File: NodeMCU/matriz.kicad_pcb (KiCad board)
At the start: 2 copper layers, 70 x 70 mm, 25 parts, among them J1 Conn_01x05, Q1 Q_NPN_CBE, Q2 Q_NPN_CBE, Q3 Q_NPN_CBE, SW1 SW_Push_Open, SW2 SW_Push, U3 NodeMCU1.0(ESP-12E)

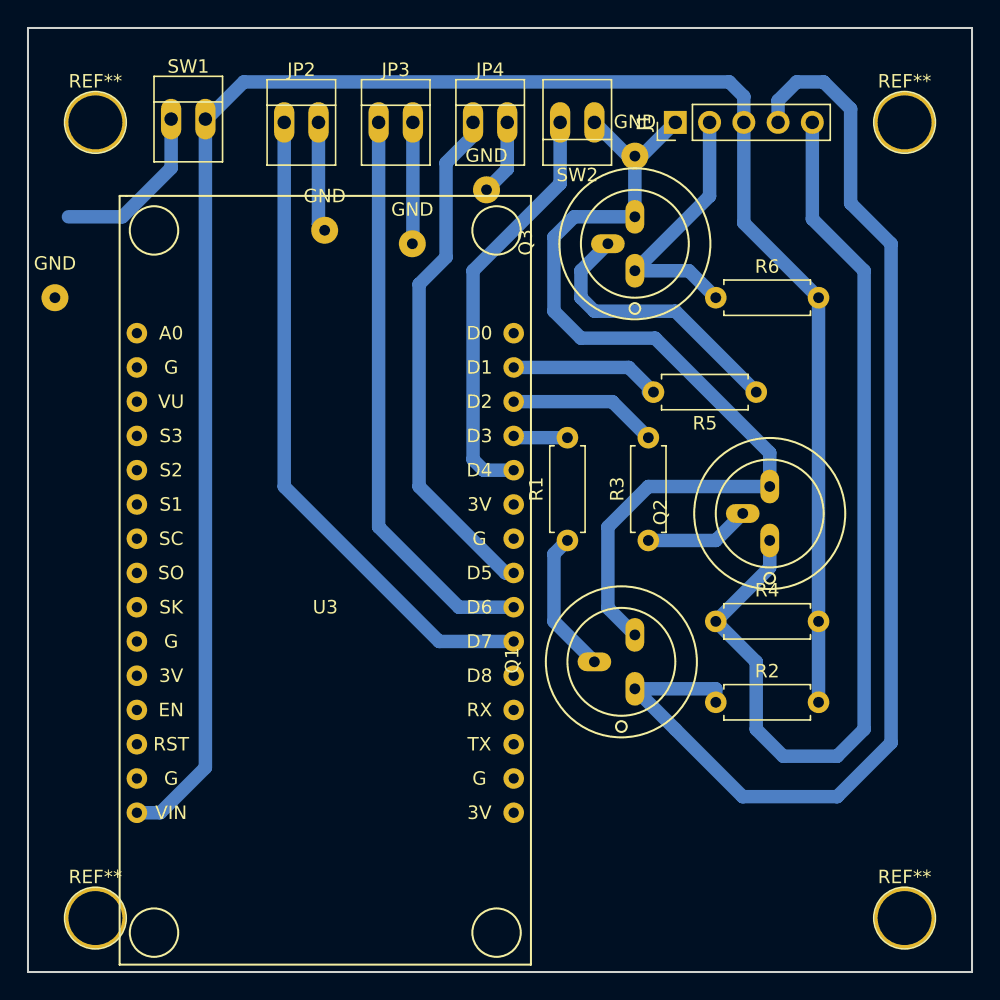
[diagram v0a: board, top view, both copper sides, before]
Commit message: Ultimos cambios
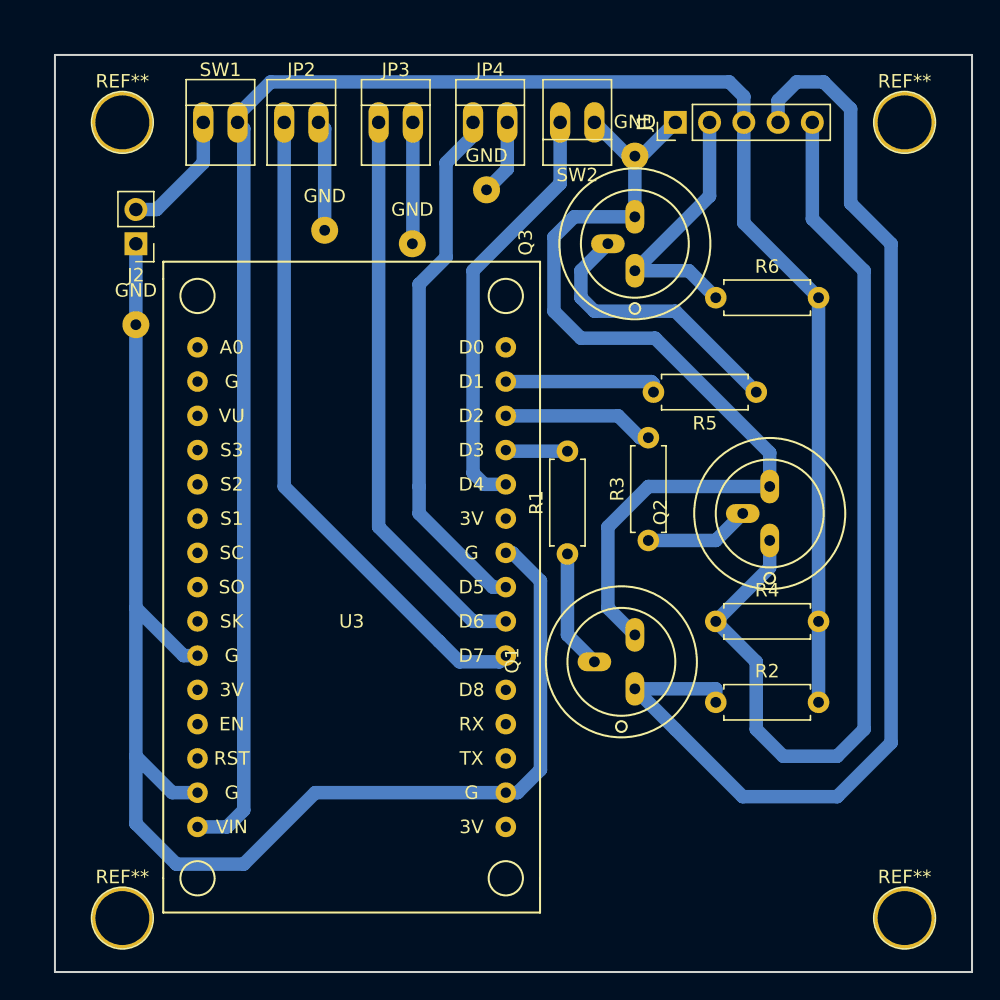
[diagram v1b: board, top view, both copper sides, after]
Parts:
- added J2: Conn_01x02, Pin_Headers:Pin_Header_Straight_1x02_Pitch2.54mm, F.Cu at (92.0, 81.0)
- U3: footprint ESP8266:NodeMCU1.0(12-E) -> lib:NodeMCU1.0(12-E)
- moved GND 6.32 mm to (92.0, 87.0)
- moved SW1 2.40 mm to (97.0, 72.0)
- moved U3 2.22 mm to (108.0, 109.0)
- moved REF** 2.00 mm to (91.0, 131.0)
- moved REF** 2.00 mm to (91.0, 72.0)
- moved R1 1.00 mm to (124.0, 104.0)
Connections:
- GND pad 1: (no net) -> /GND
- GND pad 1: GNDPWR -> /GND (x4)
- J1 pad 1: GNDPWR -> /GND
- JP2 pad 2: GNDPWR -> /GND
- JP3 pad 2: GNDPWR -> /GND
- JP4 pad 2: GNDPWR -> /GND
- Q1 pad 3: GNDPWR -> /GND
- Q2 pad 3: GNDPWR -> /GND
- Q3 pad 3: GNDPWR -> /GND
- SW1 pad 1: +5V -> /PWR
- SW2 pad 1: GNDPWR -> /GND
- U3 pad 10: Net-(U3-Pad10) -> /GND
- U3 pad 14: Net-(U3-Pad14) -> /GND
- U3 pad 17: Net-(U3-Pad17) -> /GND
- U3 pad 24: Net-(U3-Pad24) -> /GND
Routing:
- net /GND: track 0.00 -> 199.2 mm
- net GNDPWR: track 93.5 -> 0.00 mm
- net +5V: track 12.7 -> 0.00 mm
- net /PWR: track 0.00 -> 9.92 mm
- net Net-(Q1-Pad2): track 10.7 -> 8.83 mm
- net /V+: track 143.3 -> 141.9 mm
- net Net-(JP4-Pad1): track 38.3 -> 39.3 mm
- net Net-(R1-Pad2): track 4.04 -> 4.60 mm
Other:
- board size 70 x 70 mm -> 68 x 68 mm
